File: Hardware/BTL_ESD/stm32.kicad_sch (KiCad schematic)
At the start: 37 parts, among them J2 BOOT, J3 Load Program, SW2 RESET, U4 STM32F103RCTx, Y1 8MHz, Y2 32.768KHz

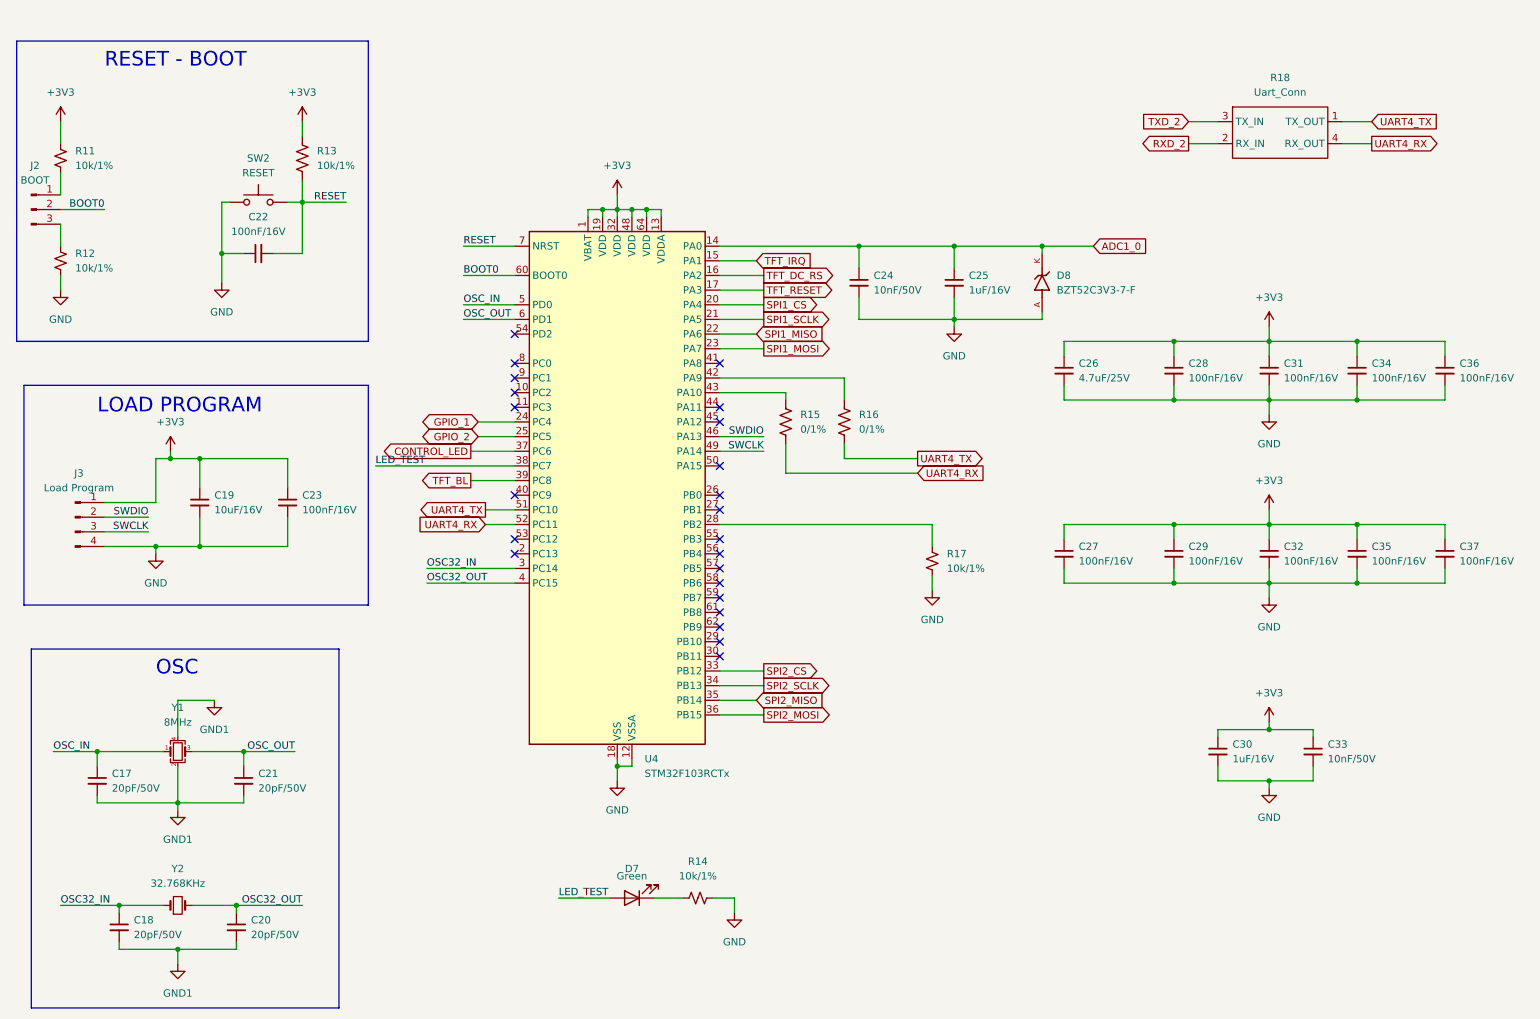
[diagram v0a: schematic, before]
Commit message: update hardware
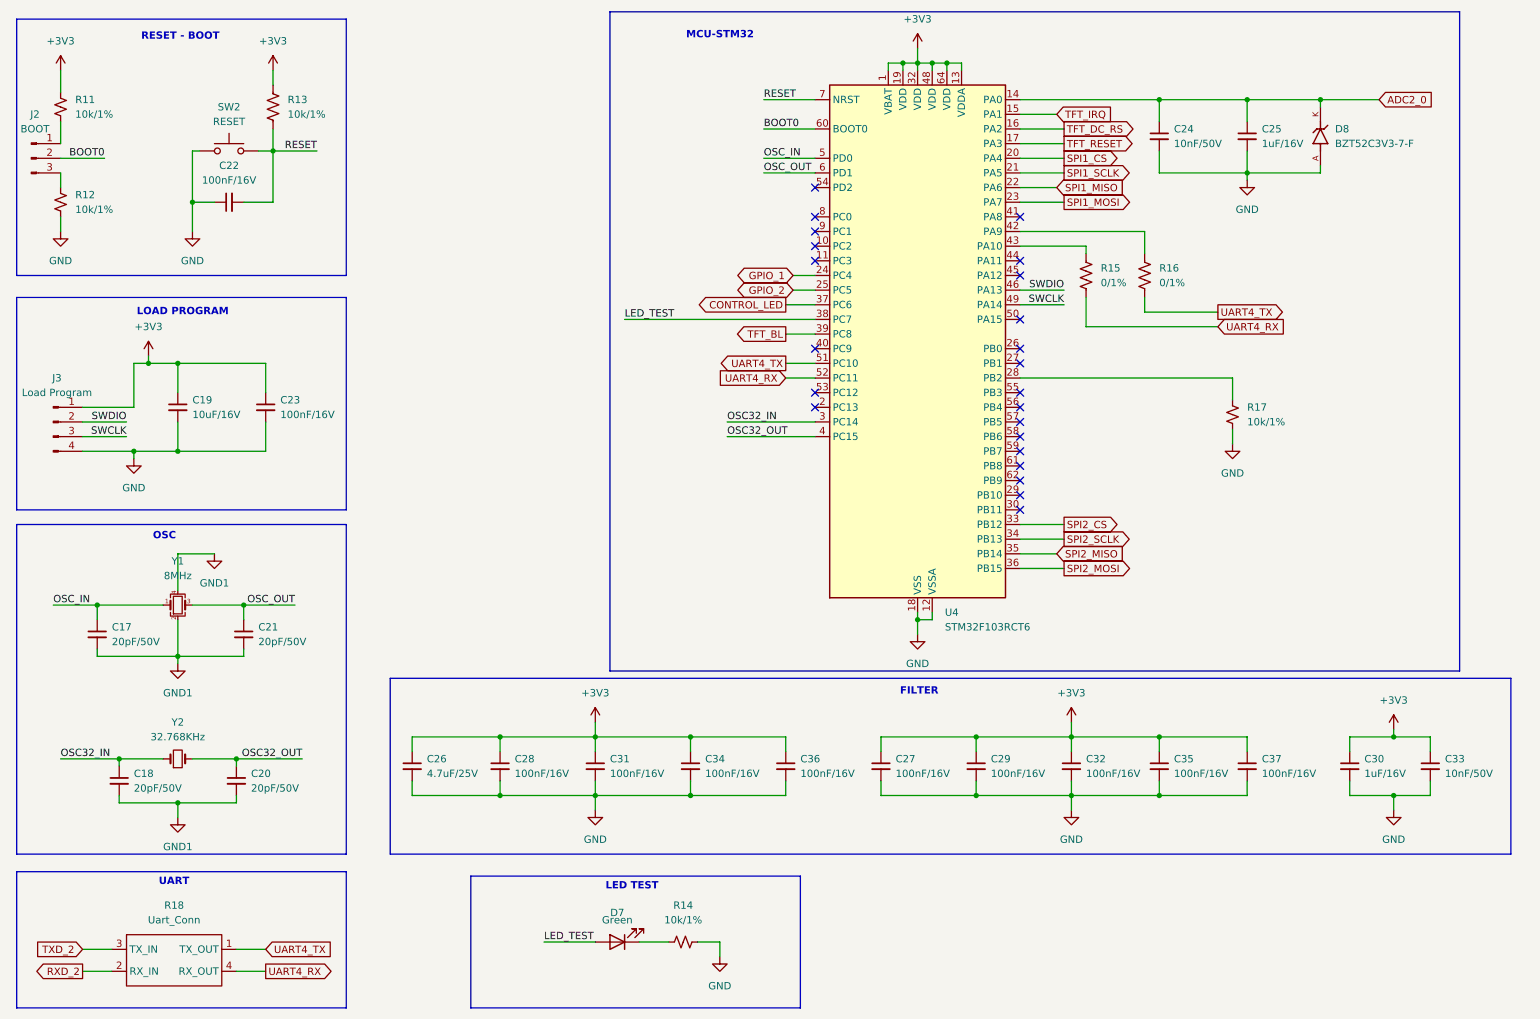
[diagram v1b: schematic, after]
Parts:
- U4: value STM32F103RCTx -> STM32F103RCT6
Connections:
- net ADC1_0 renamed ADC2_0
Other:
- note added: "FILTER"
- note added: "LED TEST"
- note added: "MCU-STM32"
- note added: "UART"
- moved on the sheet: C17, C18, C19, C20, C21, C22, C23, C24, C25, C26, C27, C28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
